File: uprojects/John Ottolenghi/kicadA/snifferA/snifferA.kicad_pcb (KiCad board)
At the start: 2 copper layers, 122.5 x 174 mm, 65 parts, among them J1 DHT22, J10 ZP07, J11 DCJ200-10-A-XX-K_REVA, J2 Conn_01x10, J3 CCS811_CJMCU, J4 Conn_01x08, J5 Conn_01x08, J6 Conn_02x18_Odd_Even, J7 Conn_01x08, J8 Conn_01x08, J9 Conn_01x08, Q1 SI4403DDY-T1-GE3, U1 MQ-131-H, U10 MQ-131-L, U12 ZE08-CH20, U13 ZP07, U14 SM4-NO2-20, U15 MQ-07, U2 MQ-135, U3 MQ-136, U4 MQ-137, U5 MQ-02, U6 MQ-04, U7 MQ-06, U8 MQ-08

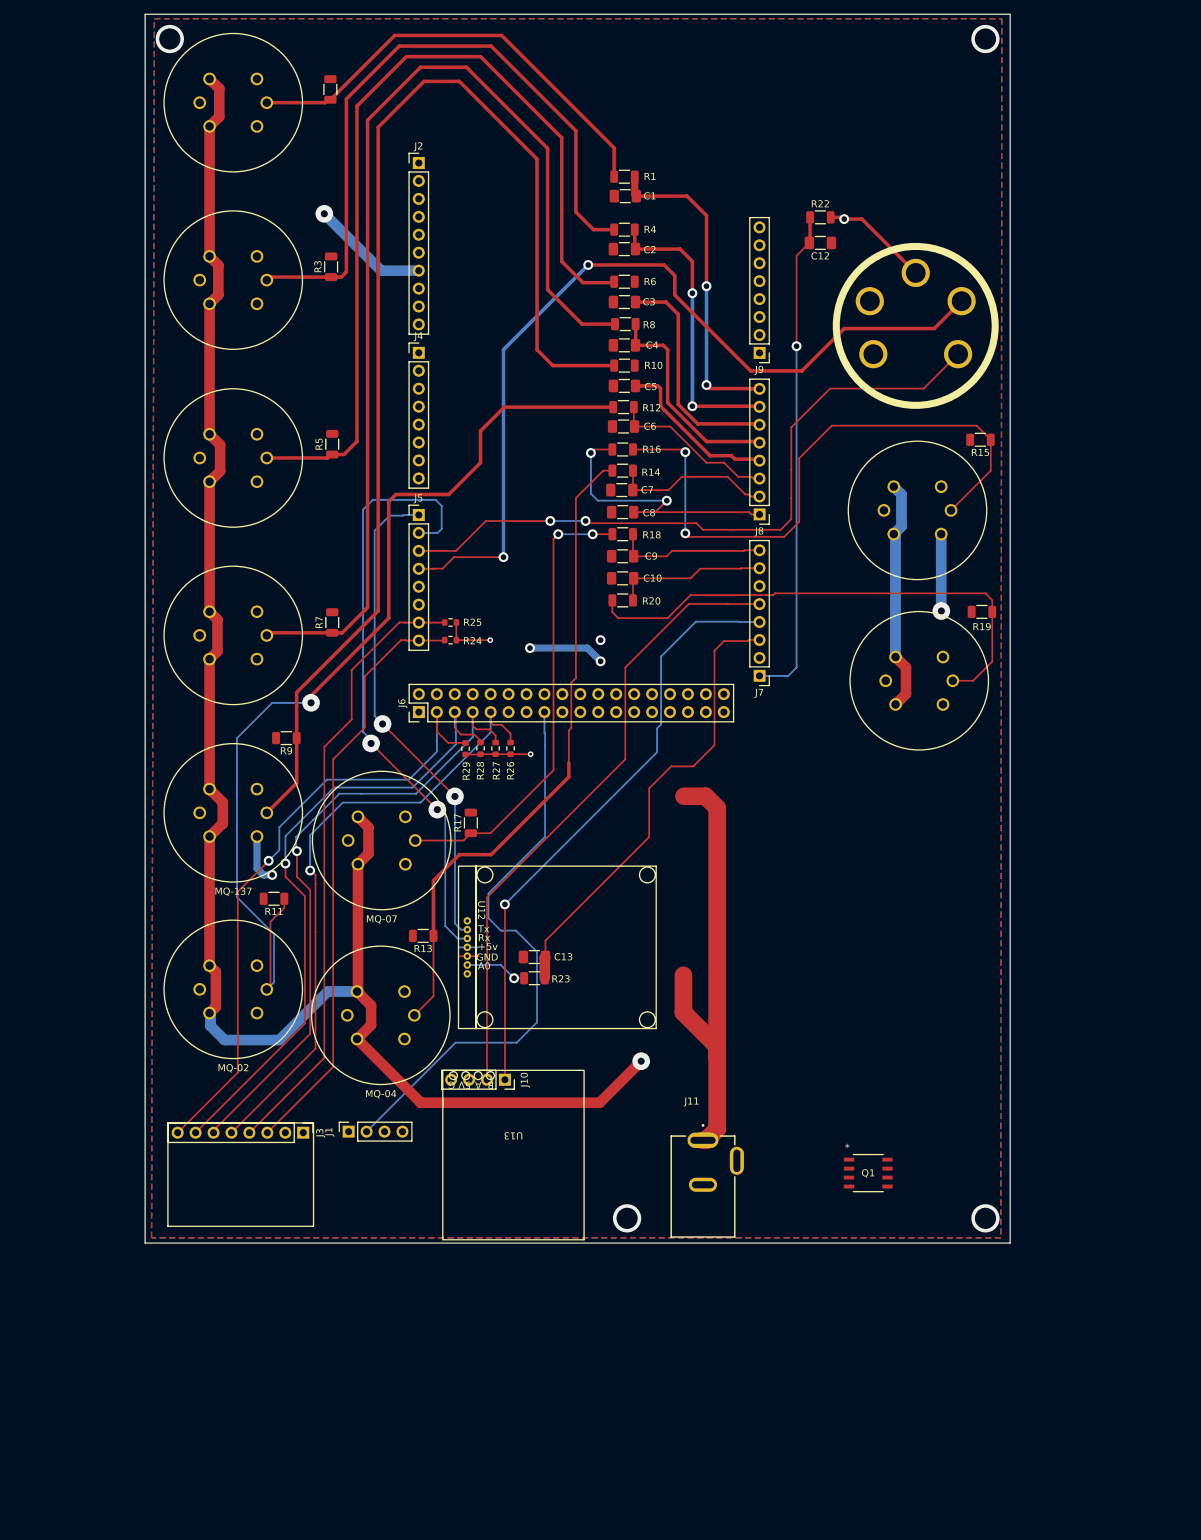
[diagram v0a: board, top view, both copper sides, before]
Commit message: Update 13 mar 2026
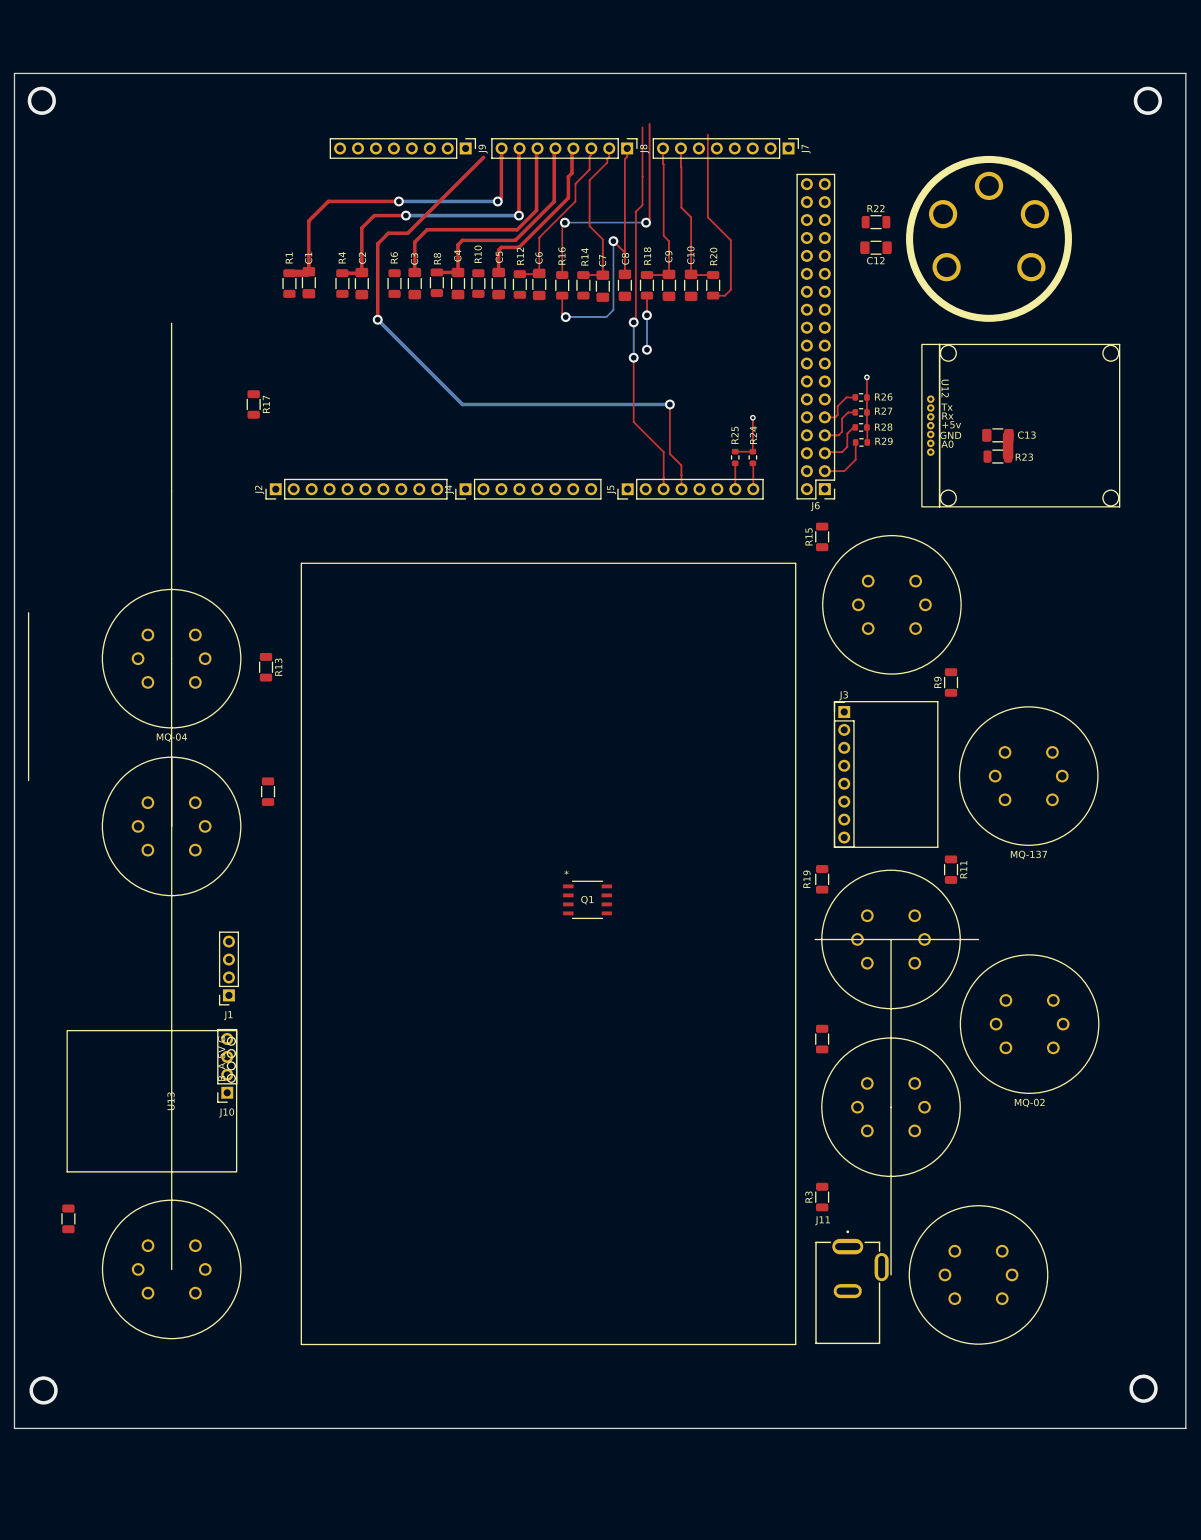
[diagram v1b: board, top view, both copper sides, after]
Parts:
- removed U15: MQ-07, MQ-X:MQ
- moved U1 176.0 mm to (157.5, 200.5)
- moved U10 170.0 mm to (145.1, 176.8)
- moved R2 151.4 mm to (135.4, 167.1)
- moved R3 149.0 mm to (135.4, 189.5)
- moved R5 115.9 mm to (28.6, 192.6)
- moved U2 115.2 mm to (43.3, 199.7)
- moved U5 112.9 mm to (164.8, 165.0)
- moved U4 112.8 mm to (164.6, 129.9)
- moved C13 98.8 mm to (160.2, 81.6)
- moved R23 98.8 mm to (160.2, 84.6)
- moved U12 98.8 mm to (150.8, 80.2)
- moved J3 97.1 mm to (138.5, 120.8), turned to 0 degrees
- moved R11 96.0 mm to (153.6, 143.1), turned to -90 degrees
- moved R9 94.5 mm to (153.6, 116.6), turned to 90 degrees
- moved J7 74.8 mm to (130.6, 41.0), turned to -90 degrees
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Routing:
- net +5VP: track 279.2 -> 0.00 mm, vias 1 -> 0
- net Net-(R10-Pad1): track 172.2 -> 0.00 mm
- net Net-(R7-Pad1): track 149.8 -> 0.00 mm
- net Net-(R11-Pad1): track 137.7 -> 0.00 mm, vias 1 -> 0
- net Net-(R5-Pad1): track 124.1 -> 0.00 mm
- net Net-(R3-Pad1): track 94.8 -> 0.00 mm
- net Net-(R13-Pad1): track 92.1 -> 0.00 mm
- net /A11-ZP07-A: track 89.2 -> 0.00 mm
- net Net-(J5-Pin_2): track 86.7 -> 0.00 mm, vias 2 -> 0
- net /A12-ZP07-B: track 85.1 -> 0.00 mm, vias 1 -> 0
- net /SDA: track 87.5 -> 3.68 mm
- net /RST: track 90.6 -> 6.93 mm, vias 1 -> 0
- net /INT: track 89.6 -> 6.77 mm, vias 1 -> 0
- net /DHT22_DATA: track 82.0 -> 0.00 mm
- net /WAK: track 88.1 -> 6.22 mm, vias 1 -> 0
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- removed copper zone on B.Cu, net +5V
- removed copper zone on F.Cu, net GND
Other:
- board size 122.5 x 174 mm -> 165.9 x 191.9 mm

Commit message: local update 14 Mar 26
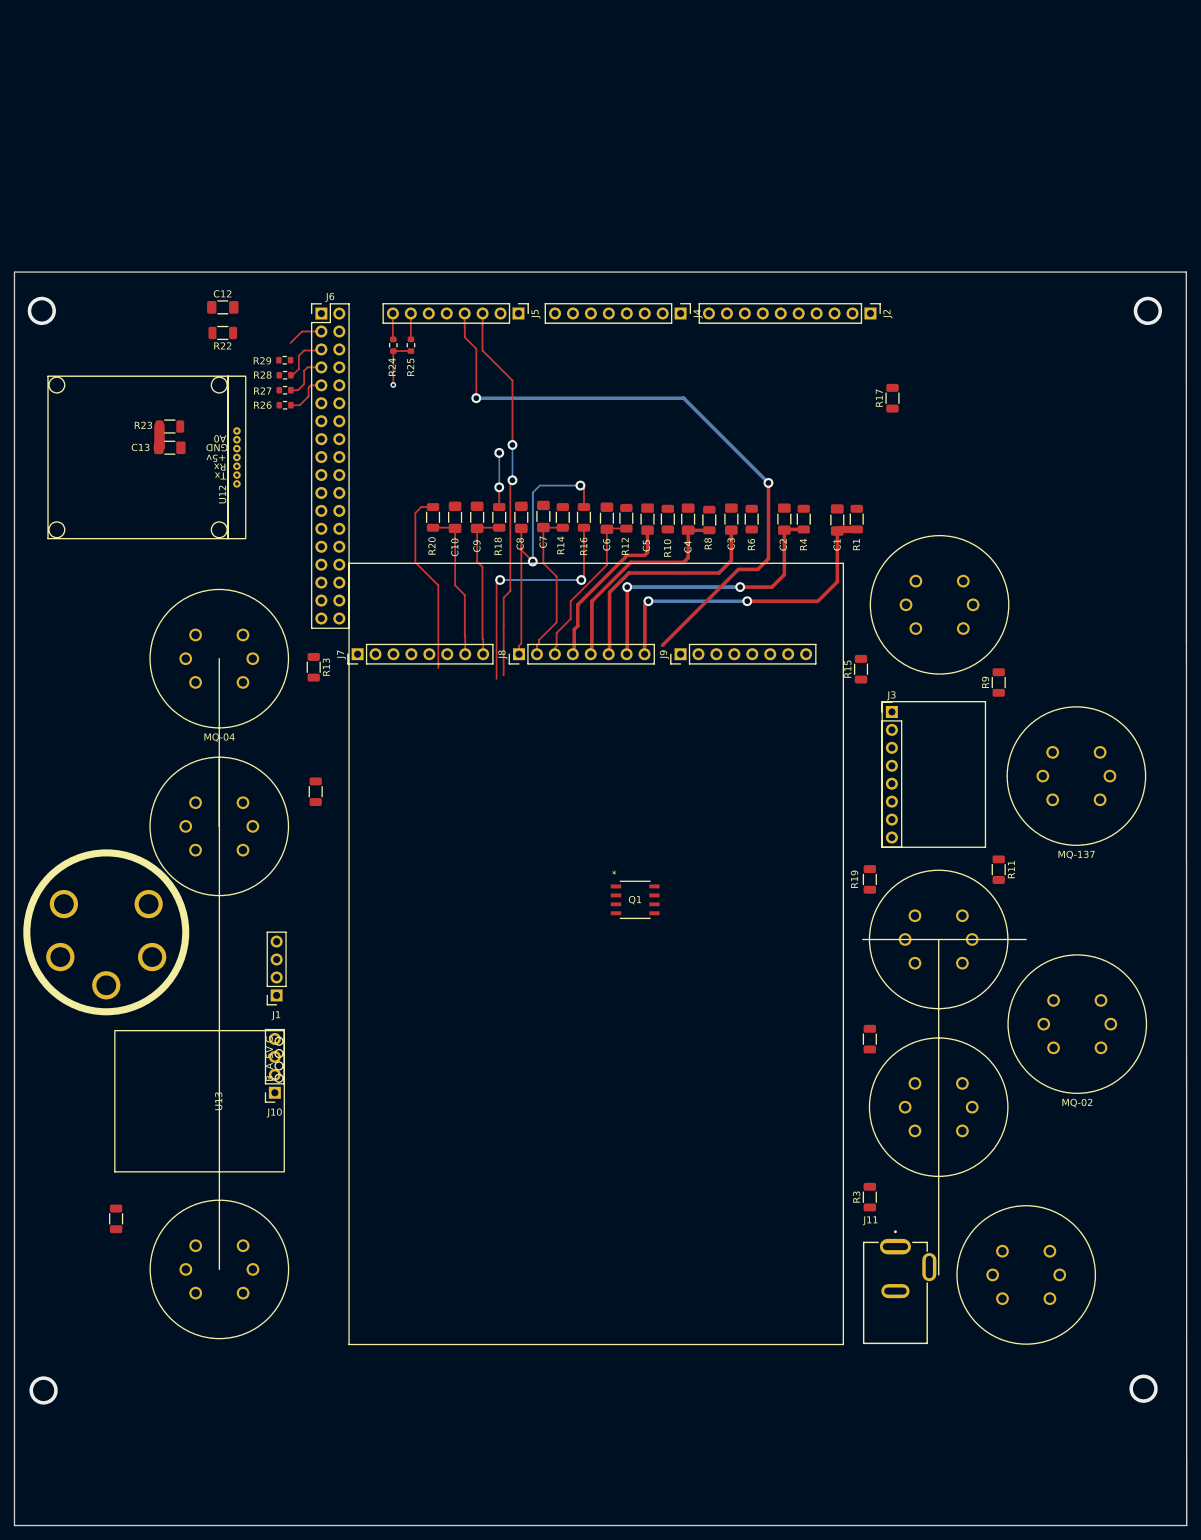
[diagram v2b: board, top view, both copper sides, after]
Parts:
- moved U14 159.0 mm to (34.0, 152.0), turned to 180 degrees
- moved R23 117.3 mm to (43.0, 80.4), turned to 180 degrees
- moved C13 117.3 mm to (43.0, 83.4), turned to 180 degrees
- moved U12 98.4 mm to (52.5, 84.8), turned to 90 degrees
- moved J7 94.1 mm to (69.6, 112.6), turned to 90 degrees
- moved R22 93.8 mm to (50.5, 67.1), turned to 0 degrees
- moved C12 92.9 mm to (50.5, 63.5), turned to 0 degrees
- moved R17 90.5 mm to (145.3, 76.4), turned to 90 degrees
- moved J2 87.8 mm to (142.2, 64.4), turned to -90 degrees
- moved R1 87.0 mm to (140.3, 93.5), turned to -90 degrees
- moved R29 82.5 mm to (59.3, 71.0), turned to 0 degrees
- moved C1 82.0 mm to (137.5, 93.6), turned to -90 degrees
- moved R28 81.9 mm to (59.3, 73.1), turned to 0 degrees
- moved R27 81.6 mm to (59.3, 75.2), turned to 0 degrees
- moved R26 81.6 mm to (59.3, 77.4), turned to 0 degrees
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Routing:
- net +3.3V: track 16.6 -> 7.30 mm, vias 2 -> 1
- net /ADD: track 7.48 -> 5.03 mm
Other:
- board size 165.9 x 191.9 mm -> 166 x 177.5 mm
